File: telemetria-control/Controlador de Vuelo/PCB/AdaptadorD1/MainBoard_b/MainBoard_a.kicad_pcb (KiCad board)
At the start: 2 copper layers, 43.2 x 43.2 mm, 7 parts, among them J1 Conn_01x04, Q1 BC548, U1 WeMos_mini

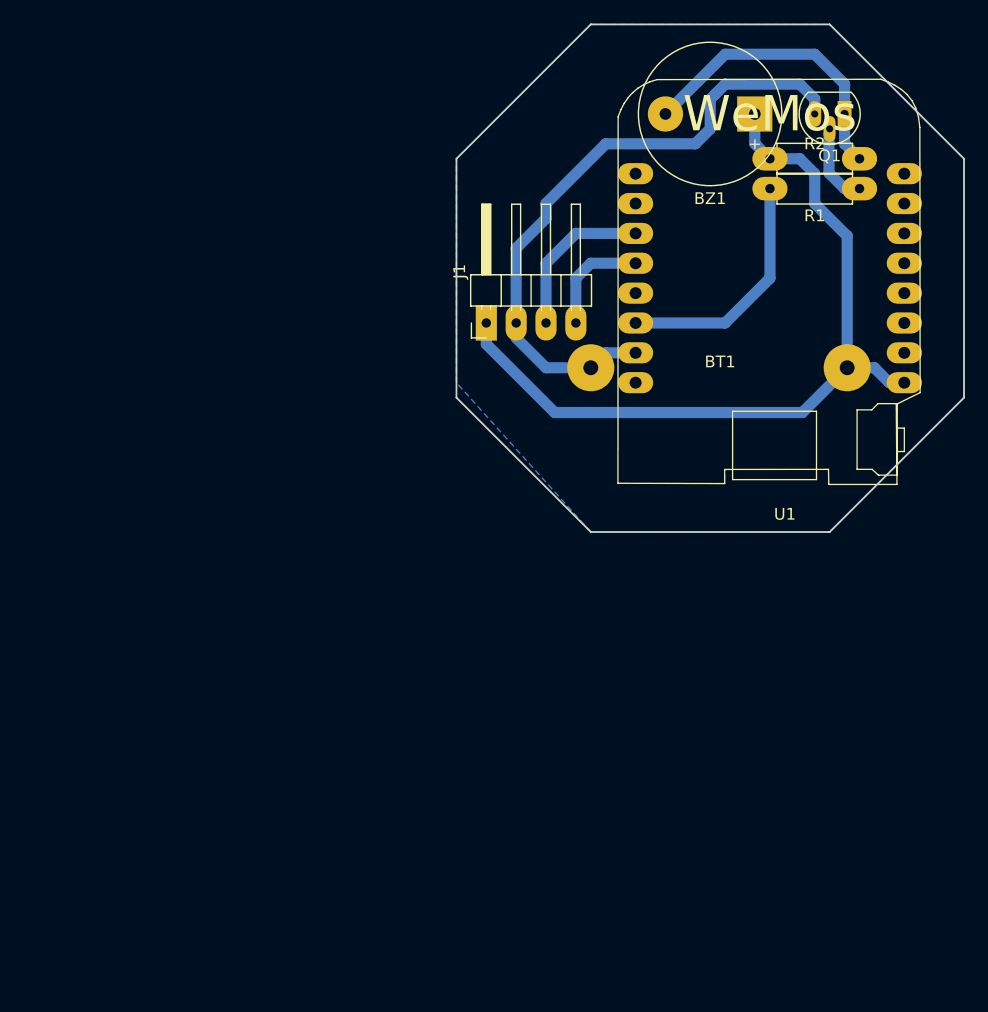
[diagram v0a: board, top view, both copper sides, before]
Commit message: Add files via upload
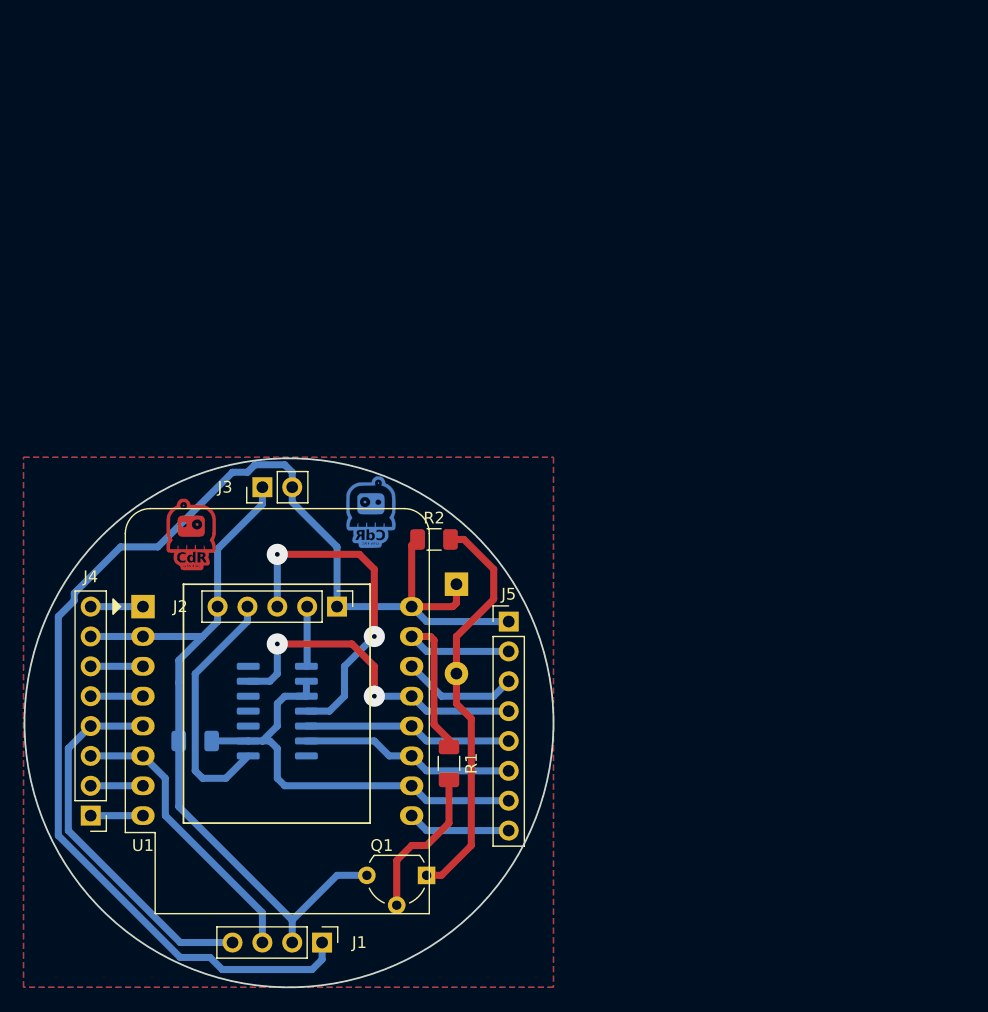
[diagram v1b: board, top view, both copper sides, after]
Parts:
- removed BT1: Battery_Cell, Componentes:Holder2032
- added ?: , kicad:logo, F.Cu at (154.9, 76.8)
- added ?: , kicad:logo, B.Cu at (140.3, 78.7)
- added J2: Conn_01x05, Connector_PinHeader_2.54mm:PinHeader_1x05_P2.54mm_Vertical, F.Cu at (152.4, 85.1)
- added J3: Conn_01x02, Connector_PinHeader_2.54mm:PinHeader_1x02_P2.54mm_Vertical, F.Cu at (146.1, 74.9)
- added J4: Conn_01x08, Connector_PinHeader_2.54mm:PinHeader_1x08_P2.54mm_Vertical, F.Cu at (131.4, 102.9)
- added J5: Conn_01x08, Connector_PinHeader_2.54mm:PinHeader_1x08_P2.54mm_Vertical, F.Cu at (167.0, 86.4)
- added R3: 10K, Resistor_SMD:R_1206_3216Metric, B.Cu at (140.3, 96.5)
- added U2: 4066, Package_SO:SOIC-14_3.9x8.7mm_P1.27mm, B.Cu at (147.3, 94.0)
- BZ1: footprint Buzzers_Beepers:Buzzer_12x9.5RM7.6 -> Buzzer_Beeper:Buzzer_12x9.5RM7.6; moved to B.Cu
- J1: footprint Pin_Headers:Pin_Header_Angled_1x04_Pitch2.54mm -> Connector_PinHeader_2.54mm:PinHeader_1x04_P2.54mm_Vertical
- Q1: footprint TO_SOT_Packages_THT:TO-92_Molded_Narrow -> Package_TO_SOT_THT:TO-92L_Wide
- R1, R2: footprint Resistors_THT:R_Axial_DIN0207_L6.3mm_D2.5mm_P7.62mm_Horizontal -> Resistor_SMD:R_1206_3216Metric
- U1: footprint wemos_d1_mini:D1_mini_board -> Module:WEMOS_D1_mini_light
- moved Q1 73.9 mm to (160.0, 108.0)
- moved R1 60.1 mm to (161.9, 98.4), turned to 90 degrees
- moved U1 59.6 mm to (135.9, 85.1)
- moved J1 54.5 mm to (151.1, 113.7), turned to 270 degrees
- moved BZ1 47.4 mm to (162.6, 83.2), turned to 270 degrees
- moved R2 43.2 mm to (160.7, 79.4)
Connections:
- U1 pad 10: Net-(U1-Pad10) -> Analog
- U1 pad 11: Net-(U1-Pad11) -> X_Sel
- U1 pad 12: Net-(U1-Pad12) -> Y_Sel
- U1 pad 13: Net-(U1-Pad13) -> Z_Sel
- U1 pad 15: Net-(U1-Pad15) -> Buzzer
- U1 pad 3: Buzzer -> Net-(J4-Pad6)
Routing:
- net 3v3: track 69.5 -> 113.1 mm
- net Analog: track 0.00 -> 36.6 mm
- net Net-(J2-Pad3): track 0.00 -> 28.8 mm, vias 0 -> 2
- net Z_Sel: track 0.00 -> 28.8 mm, vias 0 -> 2
- net SDA: track 9.42 -> 32.0 mm
- net Net-(J2-Pad4): track 0.00 -> 21.4 mm
- net X_Sel: track 0.00 -> 18.3 mm
- net Y_Sel: track 0.00 -> 17.7 mm
- net SCL: track 13.8 -> 24.5 mm
- net Net-(BZ1-Pad2): track 25.3 -> 35.6 mm
- net Net-(J5-Pad3): track 0.00 -> 10.0 mm
- net Net-(J5-Pad8): track 0.00 -> 8.78 mm
- net GND: track 54.6 -> 63.1 mm
- net Net-(Q1-Pad2): track 6.90 -> 13.3 mm
- net Net-(J2-Pad2): track 0.00 -> 5.11 mm
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- added copper zone on F.Cu, net GND
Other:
- board size 43.2 x 43.2 mm -> 45 x 45 mm
- net class Default: trace_width 0.95 -> 0.6
